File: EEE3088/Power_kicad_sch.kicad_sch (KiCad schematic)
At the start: 28 parts, among them U1 TP4056, U2 HT7533-1

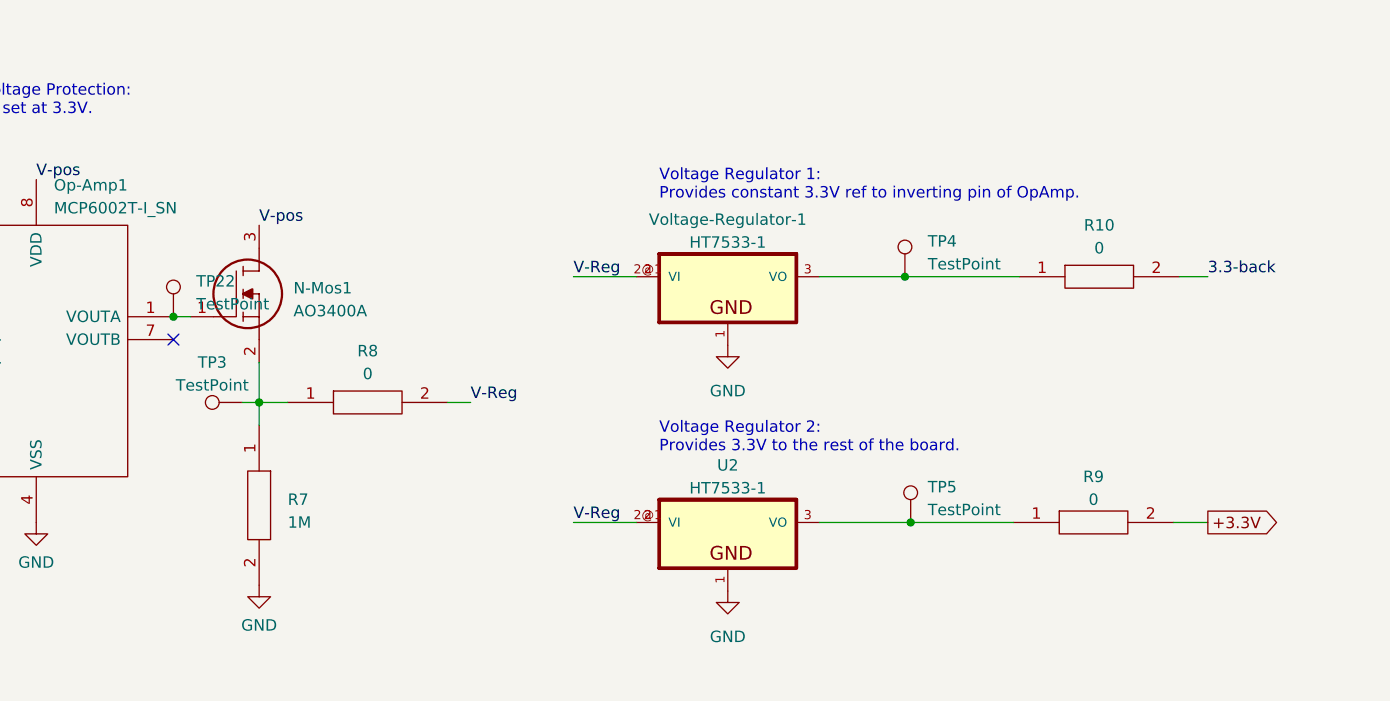
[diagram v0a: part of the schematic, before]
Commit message: Light update to power
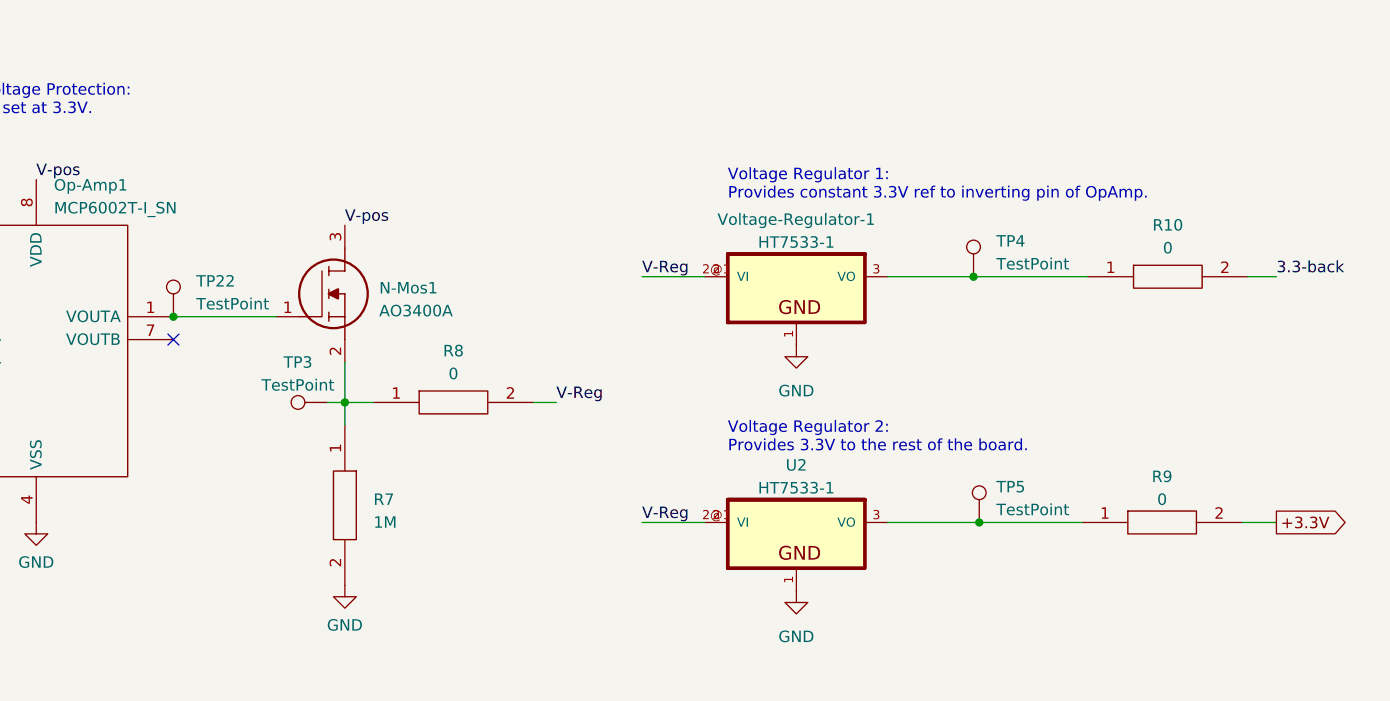
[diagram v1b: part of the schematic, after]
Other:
- moved on the sheet: N-Mos1, R10, R7, R8, R9, TP3, TP4, TP5, U2, Voltage-Regulator-1
